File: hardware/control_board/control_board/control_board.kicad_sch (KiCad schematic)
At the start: 5 parts, among them J1 Conn_02x08_Counter_Clockwise, J3 USB_B

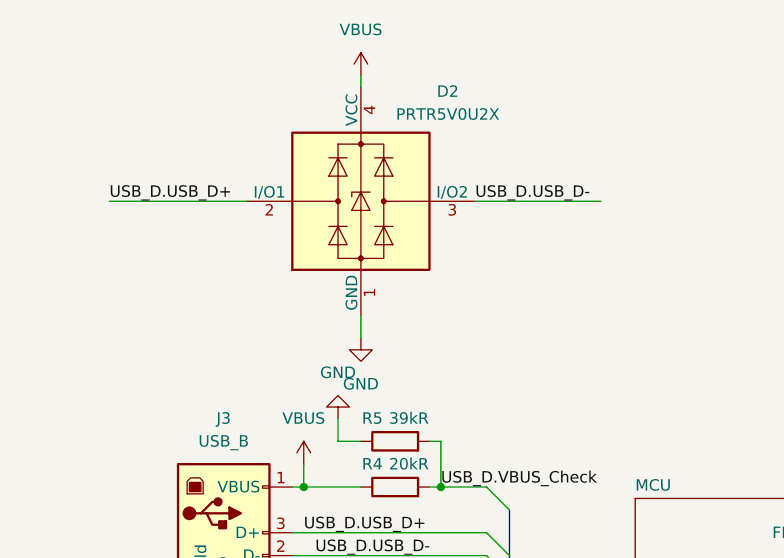
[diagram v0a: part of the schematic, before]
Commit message: feat：EEPROM原理图
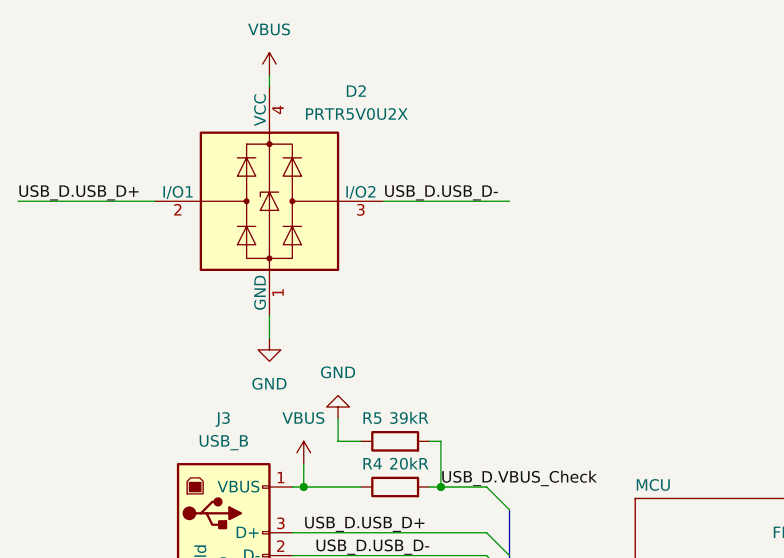
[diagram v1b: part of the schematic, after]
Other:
- moved on the sheet: D2
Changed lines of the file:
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@@
 	(wire
 		(pts
-			(xy 55.88 29.21) (xy 55.88 30.48)
+			(xy 45.72 29.21) (xy 45.72 30.48)
 		)
 		(stroke
@@
 	(wire
 		(pts
-			(xy 55.88 55.88) (xy 55.88 58.42)
+			(xy 45.72 55.88) (xy 45.72 58.42)
 		)
 		(stroke
@@
 	(wire
 		(pts
-			(xy 27.94 43.18) (xy 43.18 43.18)
+			(xy 17.78 43.18) (xy 33.02 43.18)
 		)
 		(stroke
@@
 	(wire
 		(pts
-			(xy 68.58 43.18) (xy 82.55 43.18)
+			(xy 58.42 43.18) (xy 72.39 43.18)
 		)
 		(stroke
@@
 	)
 	(label "USB_D.USB_D+"
-		(at 27.94 43.18 0)
+		(at 17.78 43.18 0)
 		(effects
 			(font
@@
 	)
 	(label "USB_D.USB_D-"
-		(at 68.58 43.18 0)
+		(at 58.42 43.18 0)
 		(effects
 			(font
@@
 	(symbol
 		(lib_id "power:VBUS")
-		(at 55.88 29.21 0)
+		(at 45.72 29.21 0)
 		(unit 1)
 		(body_style 1)
@@
 		(fields_autoplaced yes)
 		(property "Reference" "#PWR021"
-			(at 55.88 33.02 0)
+			(at 45.72 33.02 0)
 			(hide yes)
 			(show_name no)
@@
 		)
 		(property "Value" "VBUS"
-			(at 55.88 24.13 0)
+			(at 45.72 24.13 0)
 			(show_name no)
 			(do_not_autoplace no)
@@
 		)
 		(property "Footprint" ""
-			(at 55.88 29.21 0)
+			(at 45.72 29.21 0)
 			(hide yes)
 			(show_name no)
@@
 		)
 		(property "Datasheet" ""
-			(at 55.88 29.21 0)
+			(at 45.72 29.21 0)
 			(hide yes)
 			(show_name no)
@@
 		)
 		(property "Description" "Power symbol creates a global label with name \"VBUS\""
-			(at 55.88 29.21 0)
+			(at 45.72 29.21 0)
 			(hide yes)
 			(show_name no)
@@
 	(symbol
 		(lib_id "Power_Protection:PRTR5V0U2X")
-		(at 55.88 43.18 0)
+		(at 45.72 43.18 0)
 		(unit 1)
 		(body_style 1)
@@
 		(dnp no)
 		(property "Reference" "D2"
-			(at 65.532 30.988 0)
+			(at 55.372 30.988 0)
 			(show_name no)
 			(do_not_autoplace no)
@@
 		)
 		(property "Value" "PRTR5V0U2X"
-			(at 65.532 33.528 0)
+			(at 55.372 33.528 0)
 			(show_name no)
 			(do_not_autoplace no)
@@
 		)
 		(property "Footprint" "Package_TO_SOT_SMD:SOT-143"
-			(at 57.404 43.18 0)
+			(at 47.244 43.18 0)
 			(hide yes)
 			(show_name no)
@@
 		)
 		(property "Datasheet" "https://assets.nexperia.com/documents/data-sheet/PRTR5V0U2X.pdf"
-			(at 57.404 43.18 0)
+			(at 47.244 43.18 0)
 			(hide yes)
 			(show_name no)
@@
 		)
 		(property "Description" "Ultra low capacitance double rail-to-rail ESD protection diode, SOT-143"
-			(at 55.88 43.18 0)
+			(at 45.72 43.18 0)
 			(hide yes)
 			(show_name no)
@@
 		)
 		(property "KLC_S3.3" ""
-			(at 55.88 43.18 0)
+			(at 45.72 43.18 0)
 			(hide yes)
 			(show_name no)
@@
 		)
 		(property "KLC_S4.1" ""
-			(at 55.88 43.18 0)
+			(at 45.72 43.18 0)
 			(hide yes)
 			(show_name no)
@@
 	(symbol
 		(lib_id "power:GND")
-		(at 55.88 58.42 0)
+		(at 45.72 58.42 0)
 		(unit 1)
 		(body_style 1)
@@
 		(fields_autoplaced yes)
 		(property "Reference" "#PWR020"
-			(at 55.88 64.77 0)
+			(at 45.72 64.77 0)
 			(hide yes)
 			(show_name no)
@@
 		)
 		(property "Value" "GND"
-			(at 55.88 63.5 0)
+			(at 45.72 63.5 0)
 			(show_name no)
 			(do_not_autoplace no)
@@
 		)
 		(property "Footprint" ""
-			(at 55.88 58.42 0)
+			(at 45.72 58.42 0)
 			(hide yes)
 			(show_name no)
@@
 		)
 		(property "Datasheet" ""
-			(at 55.88 58.42 0)
+			(at 45.72 58.42 0)
 			(hide yes)
 			(show_name no)
@@
 		)
 		(property "Description" "Power symbol creates a global label with name \"GND\" , ground"
-			(at 55.88 58.42 0)
-			(hide yes)
-			(show_name no)
+			(at 45.72 58.42 0)
+			(hide yes)
+			(show_name no)
